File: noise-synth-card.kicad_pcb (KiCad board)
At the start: 2 copper layers, 85.1 x 53.3 mm, 104 parts, among them J1 CVpitch, J10 VCO-out, J11 Blend Out, J13 wave-select, J2 FM in, J3 PWM in, J4 power, J5 VCO-out, J6 wave-select, J7 CVpitch, J8 FM in, J9 PWM in, M1 imogen-wren-card, Q1 BC807, Q2 BC817, Q3 BC807, Q4 BC817, U1 HEF4093B, U2 TL074, U3 TL074, U4 TL074

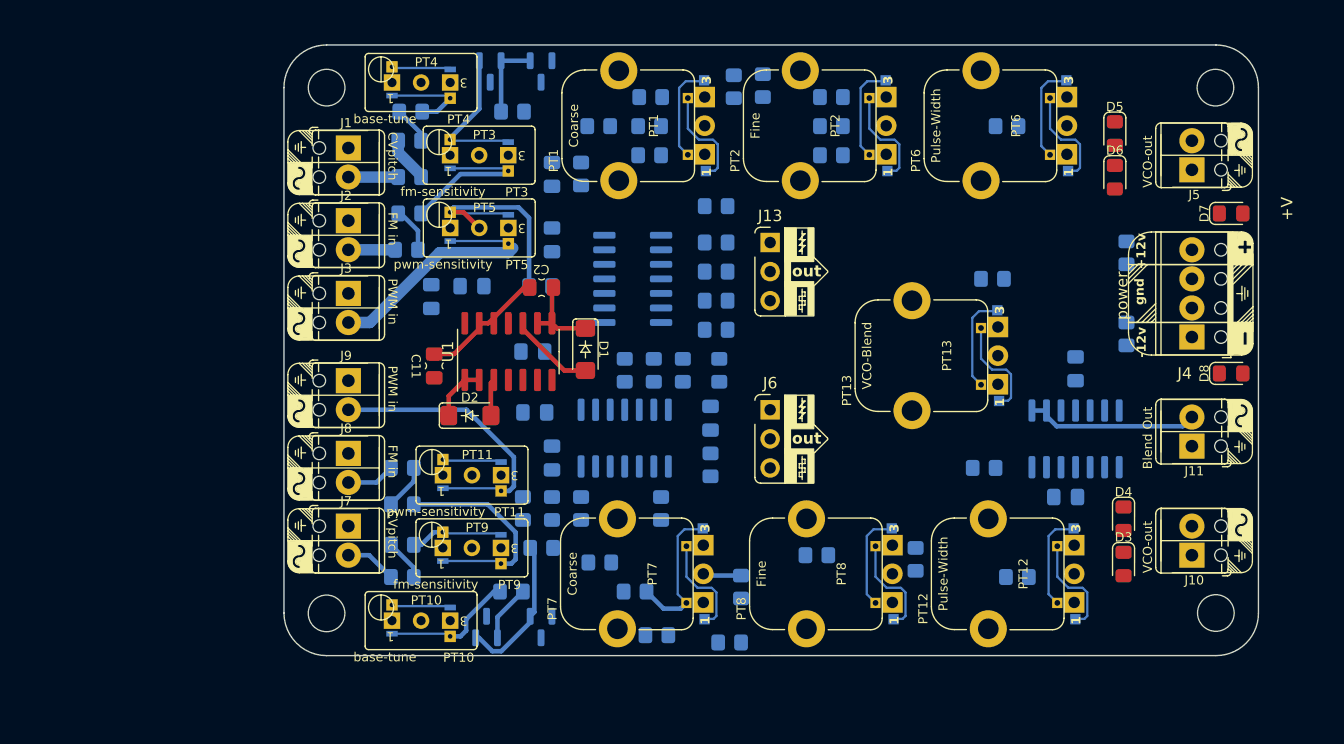
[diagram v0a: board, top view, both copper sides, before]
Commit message: layout almost finished
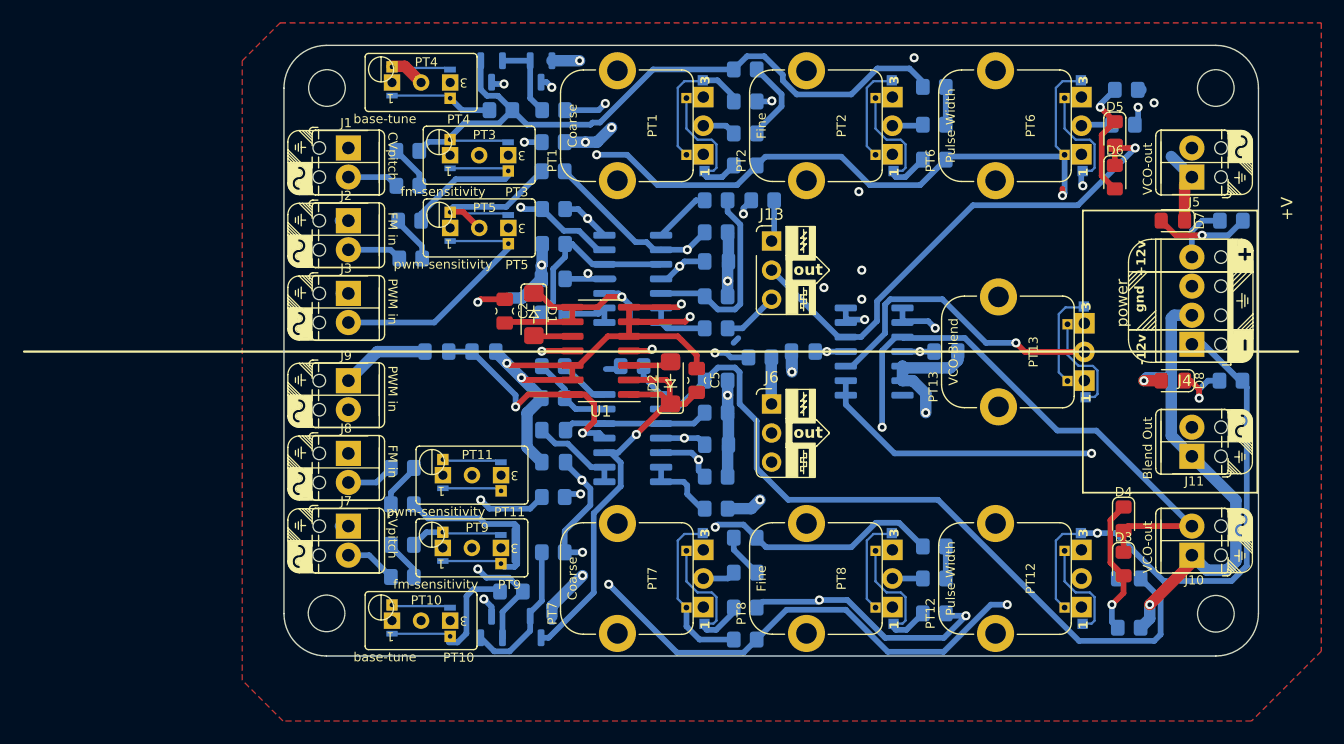
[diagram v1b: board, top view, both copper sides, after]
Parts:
- C11, M1: moved to B.Cu
- C5: moved to F.Cu
- moved C8 46.3 mm to (125.2, 85.9), turned to 180 degrees
- moved TH5 29.2 mm to (158.5, 93.2)
- moved C11 26.3 mm to (139.5, 68.3), turned to 180 degrees
- moved C1 24.0 mm to (147.0, 76.2), turned to 180 degrees
- moved R40 20.2 mm to (175.2, 53.3)
- moved U4 19.2 mm to (153.2, 76.2), turned to 0 degrees
- moved R17 19.0 mm to (125.2, 63.8), turned to 180 degrees
- moved R39 18.8 mm to (175.5, 100.3), turned to 180 degrees
- moved C12 18.0 mm to (139.5, 84.3), turned to 180 degrees
- moved D2 17.8 mm to (135.4, 78.9), turned to 90 degrees
- moved C10 16.5 mm to (159.5, 76.2), turned to 180 degrees
- moved R14 15.3 mm to (125.2, 57.9)
- moved R35 14.6 mm to (139.4, 87.1), turned to 180 degrees
- moved TH4 13.7 mm to (142.0, 51.6)
- moved R34 12.7 mm to (132.1, 77.5), turned to 0 degrees
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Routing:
- net GND: track 11.0 -> 484.2 mm, vias 0 -> 18
- net -12V: track 0.00 -> 281.3 mm, vias 0 -> 12
- net +12V: track 0.00 -> 268.9 mm, vias 0 -> 13
- net Net-(U3C--): track 0.00 -> 78.8 mm, vias 0 -> 1
- net Net-(U2C--): track 0.00 -> 63.7 mm, vias 0 -> 2
- net /VCO-saw-square-1/VCO_OUT: track 0.00 -> 59.0 mm, vias 0 -> 1
- net Net-(Q3-B): track 7.92 -> 61.3 mm, vias 0 -> 2
- net Net-(Q1-B): track 11.2 -> 61.2 mm
- net /VCO-saw-square-0/VCO_OUT: track 0.67 -> 50.6 mm, vias 0 -> 1
- net Net-(J11-signal): track 15.2 -> 55.9 mm, vias 0 -> 1
- net Net-(D1-K): track 7.54 -> 42.9 mm, vias 0 -> 2
- net Net-(D2-K): track 4.96 -> 40.0 mm, vias 0 -> 1
- net Net-(U4A-+): track 0.00 -> 26.6 mm, vias 0 -> 1
- net Net-(U4B--): track 0.00 -> 23.0 mm, vias 0 -> 1
- net Net-(U3D-+): track 0.00 -> 21.0 mm, vias 0 -> 1
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- added copper zone on F.Cu, net GND
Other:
- copper layers 2 -> 4
